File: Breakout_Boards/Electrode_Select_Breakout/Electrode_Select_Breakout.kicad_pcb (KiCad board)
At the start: 2 copper layers, 36.3 x 46.2 mm, 3 parts, among them J1 Conn_01x08_Socket, J2 2xRJ_45, J3 Conn_01x08_Socket

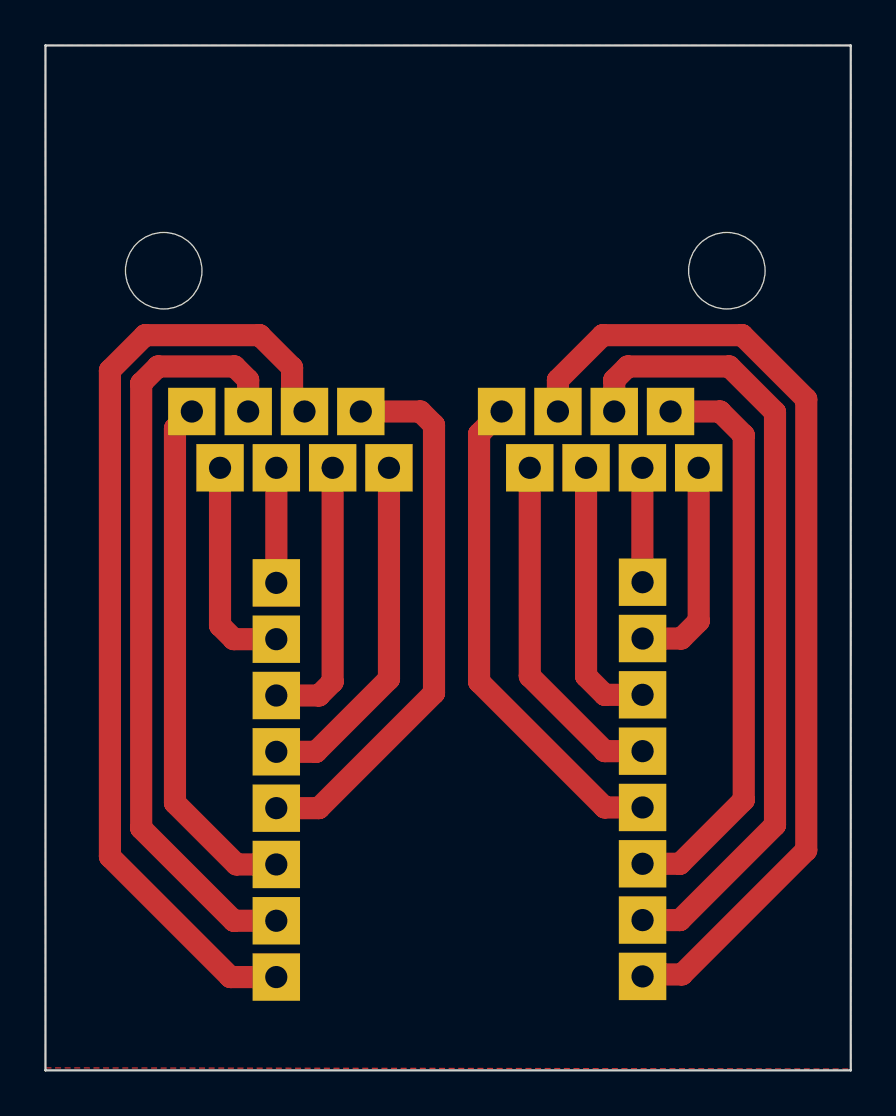
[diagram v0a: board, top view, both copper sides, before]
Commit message: Push Electrode_Breakout to Git
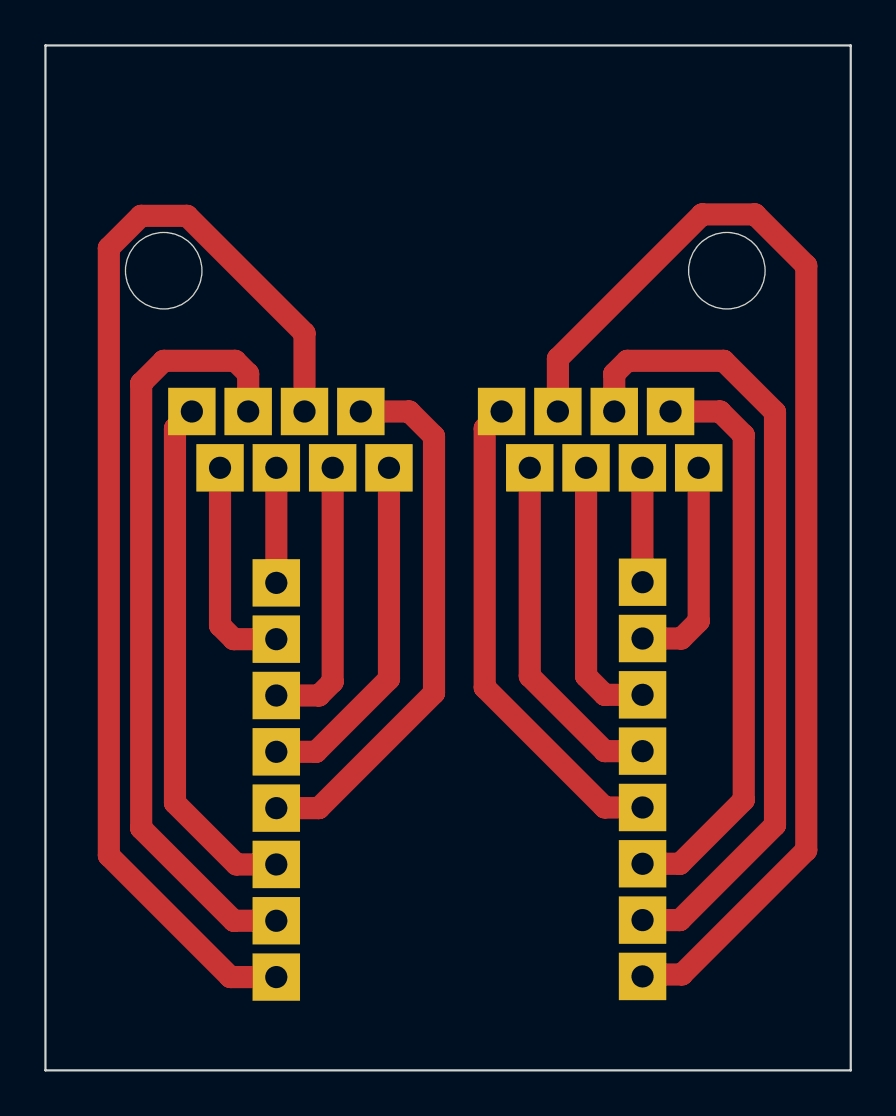
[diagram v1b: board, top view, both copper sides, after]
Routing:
- net /CH8_1: track 43.7 -> 52.4 mm
- net /CH8_2: track 44.8 -> 53.4 mm
- removed copper zone on F.Cu, net (none)
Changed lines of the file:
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@@
     (pad_to_mask_clearance 0)
     (pcbplotparams
-      (layerselection 0x0000000_7fffffff)
+      (layerselection 0x0001000_7fffffff)
       (plot_on_all_layers_selection 0x0000000_00000000)
       (disableapertmacros false)
@@
   (segment (start 21.844 28.448) (end 25.226 31.83) (width 1) (layer "F.Cu") (net 8))
   (segment (start 21.844 19.05) (end 21.844 28.448) (width 1) (layer "F.Cu") (net 8))
-  (segment (start 14.224 16.51) (end 16.914 16.51) (width 1) (layer "F.Cu") (net 9))
-  (segment (start 16.914 16.51) (end 17.526 17.122) (width 1) (layer "F.Cu") (net 9))
-  (segment (start 17.526 17.122) (end 17.526 29.21) (width 1) (layer "F.Cu") (net 9))
+  (segment (start 16.4084 16.51) (end 17.526 17.6276) (width 1) (layer "F.Cu") (net 9))
+  (segment (start 14.224 16.51) (end 16.4084 16.51) (width 1) (layer "F.Cu") (net 9))
   (segment (start 12.336 34.4) (end 10.412 34.4) (width 1) (layer "F.Cu") (net 9))
+  (segment (start 17.526 17.6276) (end 17.526 29.21) (width 1) (layer "F.Cu") (net 9))
   (segment (start 17.526 29.21) (end 12.336 34.4) (width 1) (layer "F.Cu") (net 9))
+  (segment (start 20.574 16.51) (end 19.812 17.272) (width 1) (layer "F.Cu") (net 10))
   (segment (start 25.226 34.37) (end 26.932 34.37) (width 1) (layer "F.Cu") (net 10))
-  (segment (start 19.558 28.702) (end 25.226 34.37) (width 1) (layer "F.Cu") (net 10))
-  (segment (start 19.558 17.526) (end 19.558 28.702) (width 1) (layer "F.Cu") (net 10))
-  (segment (start 20.574 16.51) (end 19.558 17.526) (width 1) (layer "F.Cu") (net 10))
+  (segment (start 19.812 17.272) (end 19.812 28.956) (width 1) (layer "F.Cu") (net 10))
+  (segment (start 19.812 28.956) (end 25.226 34.37) (width 1) (layer "F.Cu") (net 10))
+  (segment (start 5.842 34.167) (end 8.615 36.94) (width 1) (layer "F.Cu") (net 11))
   (segment (start 5.842 17.272) (end 5.842 34.167) (width 1) (layer "F.Cu") (net 11))
+  (segment (start 6.604 16.51) (end 5.842 17.272) (width 1) (layer "F.Cu") (net 11))
   (segment (start 8.615 36.94) (end 10.412 36.94) (width 1) (layer "F.Cu") (net 11))
-  (segment (start 6.604 16.51) (end 5.842 17.272) (width 1) (layer "F.Cu") (net 11))
-  (segment (start 5.842 34.167) (end 8.615 36.94) (width 1) (layer "F.Cu") (net 11))
+  (segment (start 5.334 14.224) (end 4.318 15.24) (width 1) (layer "F.Cu") (net 12))
+  (segment (start 8.5598 14.224) (end 5.334 14.224) (width 1) (layer "F.Cu") (net 12))
+  (segment (start 4.318 35.306) (end 8.492 39.48) (width 1) (layer "F.Cu") (net 12))
+  (segment (start 9.144 14.8082) (end 8.5598 14.224) (width 1) (layer "F.Cu") (net 12))
+  (segment (start 8.492 39.48) (end 10.412 39.48) (width 1) (layer "F.Cu") (net 12))
   (segment (start 4.318 15.24) (end 4.318 35.306) (width 1) (layer "F.Cu") (net 12))
-  (segment (start 8.532 14.478) (end 5.08 14.478) (width 1) (layer "F.Cu") (net 12))
-  (segment (start 9.144 16.51) (end 9.144 15.09) (width 1) (layer "F.Cu") (net 12))
-  (segment (start 8.492 39.48) (end 10.412 39.48) (width 1) (layer "F.Cu") (net 12))
-  (segment (start 5.08 14.478) (end 4.318 15.24) (width 1) (layer "F.Cu") (net 12))
-  (segment (start 4.318 35.306) (end 8.492 39.48) (width 1) (layer "F.Cu") (net 12))
-  (segment (start 9.144 15.09) (end 8.532 14.478) (width 1) (layer "F.Cu") (net 12))
-  (segment (start 2.908 14.655959) (end 2.908 36.586) (width 1) (layer "F.Cu") (net 13))
-  (segment (start 11.124 16.458) (end 11.124 14.53) (width 1) (layer "F.Cu") (net 13))
-  (segment (start 11.124 14.53) (end 9.662 13.068) (width 1) (layer "F.Cu") (net 13))
-  (segment (start 11.684 16.51) (end 11.176 16.51) (width 1) (layer "F.Cu") (net 13))
+  (segment (start 9.144 16.51) (end 9.144 14.8082) (width 1) (layer "F.Cu") (net 12))
+  (segment (start 11.684 12.9794) (end 6.3896 7.685) (width 1) (layer "F.Cu") (net 13))
+  (segment (start 11.684 16.51) (end 11.684 12.9794) (width 1) (layer "F.Cu") (net 13))
   (segment (start 8.342 42.02) (end 10.412 42.02) (width 1) (layer "F.Cu") (net 13))
-  (segment (start 2.908 36.586) (end 8.342 42.02) (width 1) (layer "F.Cu") (net 13))
-  (segment (start 4.495958 13.068) (end 2.908 14.655959) (width 1) (layer "F.Cu") (net 13))
-  (segment (start 9.662 13.068) (end 4.495958 13.068) (width 1) (layer "F.Cu") (net 13))
-  (segment (start 11.176 16.51) (end 11.124 16.458) (width 1) (layer "F.Cu") (net 13))
-  (segment (start 25.136 13.068) (end 23.114 15.09) (width 1) (layer "F.Cu") (net 14))
+  (segment (start 2.859 9.134821) (end 2.859 36.537) (width 1) (layer "F.Cu") (net 13))
+  (segment (start 2.859 36.537) (end 8.342 42.02) (width 1) (layer "F.Cu") (net 13))
+  (segment (start 4.308821 7.685) (end 2.859 9.134821) (width 1) (layer "F.Cu") (net 13))
+  (segment (start 6.3896 7.685) (end 4.308821 7.685) (width 1) (layer "F.Cu") (net 13))
+  (segment (start 34.316 36.296) (end 34.316 9.932) (width 1) (layer "F.Cu") (net 14))
+  (segment (start 26.932 41.99) (end 26.932 41.902) (width 1) (layer "F.Cu") (net 14))
+  (segment (start 28.71 41.902) (end 34.316 36.296) (width 1) (layer "F.Cu") (net 14))
+  (segment (start 23.114 14.12491) (end 23.114 16.51) (width 1) (layer "F.Cu") (net 14))
+  (segment (start 34.316 9.932) (end 32.004 7.62) (width 1) (layer "F.Cu") (net 14))
+  (segment (start 32.004 7.62) (end 29.61891 7.62) (width 1) (layer "F.Cu") (net 14))
   (segment (start 26.932 41.902) (end 28.71 41.902) (width 1) (layer "F.Cu") (net 14))
-  (segment (start 26.932 41.99) (end 26.932 41.902) (width 1) (layer "F.Cu") (net 14))
-  (segment (start 23.114 15.09) (end 23.114 16.51) (width 1) (layer "F.Cu") (net 14))
-  (segment (start 28.71 41.902) (end 34.316 36.296) (width 1) (layer "F.Cu") (net 14))
-  (segment (start 34.316 36.296) (end 34.316 15.953917) (width 1) (layer "F.Cu") (net 14))
-  (segment (start 34.316 15.953917) (end 31.430083 13.068) (width 1) (layer "F.Cu") (net 14))
-  (segment (start 31.430083 13.068) (end 25.136 13.068) (width 1) (layer "F.Cu") (net 14))
-  (segment (start 26.266 14.478) (end 25.654 15.09) (width 1) (layer "F.Cu") (net 15))
+  (segment (start 29.61891 7.62) (end 23.114 14.12491) (width 1) (layer "F.Cu") (net 14))
   (segment (start 28.622 39.45) (end 32.906 35.166) (width 1) (layer "F.Cu") (net 15))
-  (segment (start 32.906 16.537958) (end 30.846042 14.478) (width 1) (layer "F.Cu") (net 15))
+  (segment (start 30.592042 14.224) (end 26.2382 14.224) (width 1) (layer "F.Cu") (net 15))
   (segment (start 26.932 39.45) (end 28.622 39.45) (width 1) (layer "F.Cu") (net 15))
-  (segment (start 25.654 15.09) (end 25.654 16.51) (width 1) (layer "F.Cu") (net 15))
+  (segment (start 32.906 16.537958) (end 30.592042 14.224) (width 1) (layer "F.Cu") (net 15))
   (segment (start 32.906 35.166) (end 32.906 16.537958) (width 1) (layer "F.Cu") (net 15))
-  (segment (start 30.846042 14.478) (end 26.266 14.478) (width 1) (layer "F.Cu") (net 15))
+  (segment (start 26.2382 14.224) (end 25.654 14.8082) (width 1) (layer "F.Cu") (net 15))
+  (segment (start 25.654 14.8082) (end 25.654 16.51) (width 1) (layer "F.Cu") (net 15))
   (segment (start 28.622 36.91) (end 31.496 34.036) (width 1) (layer "F.Cu") (net 16))
   (segment (start 30.428 16.51) (end 28.194 16.51) (width 1) (layer "F.Cu") (net 16))
@@
   (segment (start 31.496 17.578) (end 30.428 16.51) (width 1) (layer "F.Cu") (net 16))
   (segment (start 26.932 36.91) (end 28.622 36.91) (width 1) (layer "F.Cu") (net 16))
-  (zone (net 0) (net_name "") (layer "F.Cu") (hatch edge 0.5)
-    (connect_pads (clearance 0.41))
-    (min_thickness 0.41) (filled_areas_thickness no)
-    (fill yes (thermal_gap 0.41) (thermal_bridge_width 1) (island_removal_mode 1) (island_area_min 10))
-    (polygon
-      (pts
-        (xy 0 0)
-        (xy 0 46.116)
-        (xy 36.322 46.1668)
-        (xy 36.322 0)
-      )
-    )
-  )
 )
